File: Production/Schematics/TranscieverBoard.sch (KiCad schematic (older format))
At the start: 6 parts, among them J1 5-1814400-1, J2 Conn_01x10_Male, J3 Conn_01x10_Male, J4 Conn_01x10_Male, J5 Conn_01x10_Male, U1 MAX7037EGL+

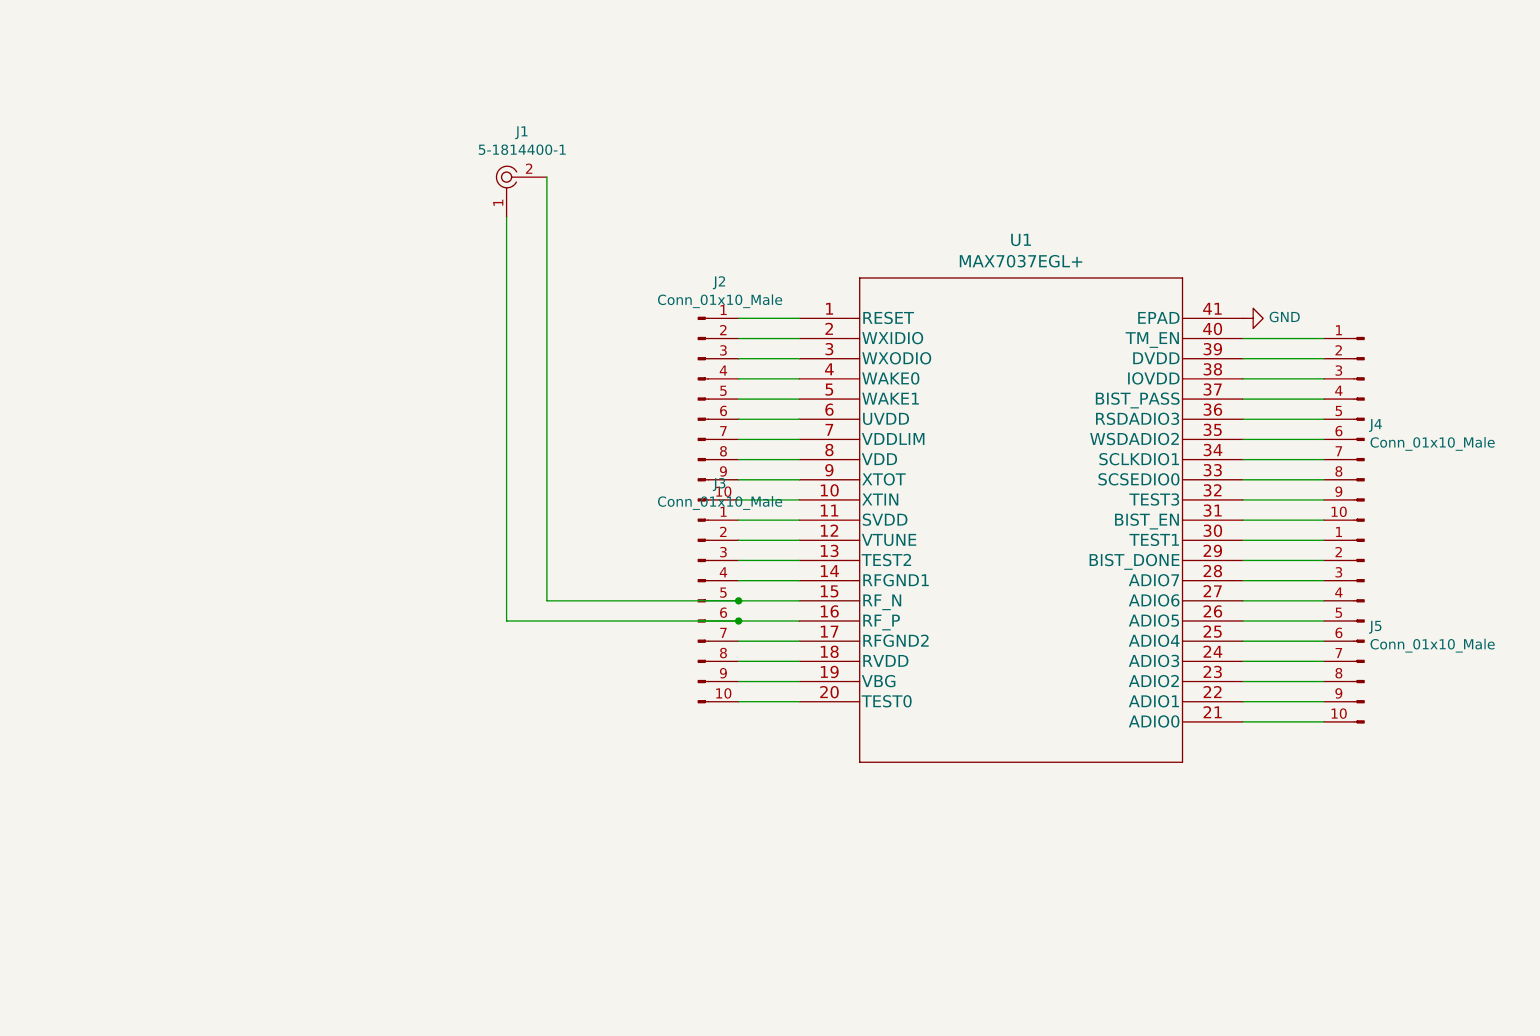
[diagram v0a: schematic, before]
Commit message: PCB Design update
PCB schematic update
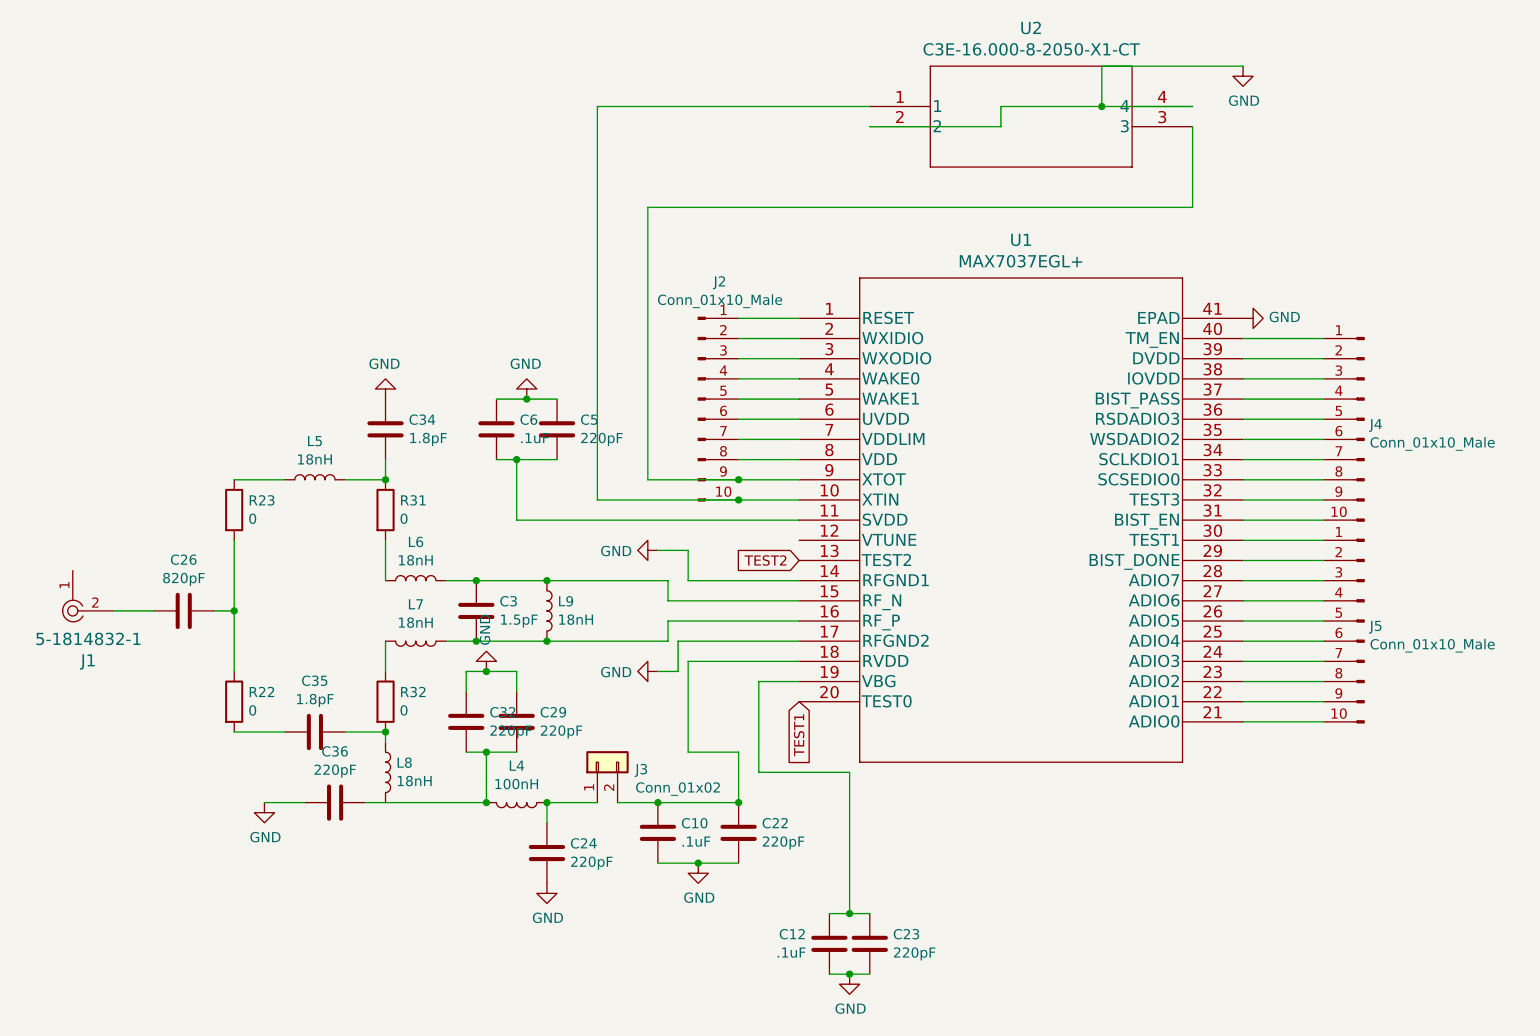
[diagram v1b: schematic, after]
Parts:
- removed J1: 5-1814400-1, digikey-footprints:RF_SMA_RightAngle_5-1814400-1, symbol dk_Coaxial-Connectors-RF:5-1814400-1
- removed J3: Conn_01x10_Male, Connector_PinHeader_2.54mm:PinHeader_1x10_P2.54mm_Vertical, symbol Connector:Conn_01x10_Male
- added C10, C12, C6: .1uF, Capacitor_SMD:C_0603_1608Metric, symbol Device:C
- added C22, C23, C24, C29, C32, C36, C5: 220pF, Capacitor_SMD:C_0402_1005Metric, symbol Device:C
- added C26: 820pF, Capacitor_SMD:C_0603_1608Metric, symbol Device:C
- added C3: 1.5pF, Capacitor_SMD:C_0402_1005Metric, symbol Device:C
- added C34, C35: 1.8pF, Capacitor_SMD:C_0402_1005Metric, symbol Device:C
- added J1: 5-1814832-1, digikey-footprints:RF_SMA_Vertical_5-1814832-1, symbol dk_Coaxial-Connectors-RF:5-1814832-1
- added J3: Conn_01x02, Connector_PinHeader_2.54mm:PinHeader_1x02_P2.54mm_Vertical, symbol Connector_Generic:Conn_01x02
- added L4: 100nH, Inductor_SMD:L_0402_1005Metric, symbol Device:L
- added L5, L6, L7, L8, L9: 18nH, Inductor_SMD:L_0402_1005Metric, symbol Device:L
- added R22, R23, R31, R32: 0, Resistor_SMD:R_0402_1005Metric, symbol Device:R
- added U2: C3E-16.000-8-2050-X1-CT, ul_C3E-16-000-8-2050-X1-CT:C3E-16.000-8-2050-X1-CT, symbol ul_C3E-16-000-8-2050-X1-CT:C3E-16.000-8-2050-X1-CT
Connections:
- net GND: now also U1.14 (RFGND1), U1.17 (RFGND2), C10.2, C12.2, C22.2, C23.2, C24.2, C29.1, C32.1, C34.2, C36.2, C5.1, C6.1, U2.2, U2.4
- net at J2.10 (Pin_10), U1.10 (XTIN): now also U2.1
- net at U1.11 (SVDD): now also C5.2, C6.2
- net TEST2: now reaches U1.13 (TEST2)
- net at U1.15 (RF_N): now also C3.1, L6.2, L9.1
- net at U1.16 (RF_P): now also C3.2, L7.1, L9.2
- net at U1.18 (RVDD): now also C10.1, C22.1, J3.2 (Pin_2)
- net at U1.19 (VBG): now also C12.1, C23.1
- net TEST1: now reaches U1.20 (TEST0)
- net at J2.9 (Pin_9), U1.9 (XTOT): now also U2.3
- new net: C26.2, J1.2
- new net: L6.1, R31.2
- new net: L7.2, R32.1
- new net: C34.1, L5.2, R31.1
- new net: C35.1, L8.1, R32.2
- new net: L5.1, R23.1
- new net: C26.1, R22.1, R23.2
- new net: C35.2, R22.2
- new net: C29.2, C32.2, C36.1, L4.2, L8.2
- new net: C24.1, J3.1 (Pin_1), L4.1
